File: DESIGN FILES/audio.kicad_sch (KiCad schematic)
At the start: 22 parts, among them J501 PJ-342B-TX-SMT, J502 PJ-342B-TX-SMT, J503 PJ-342B-TX-SMT, U501 WM8978CGEFL_RV

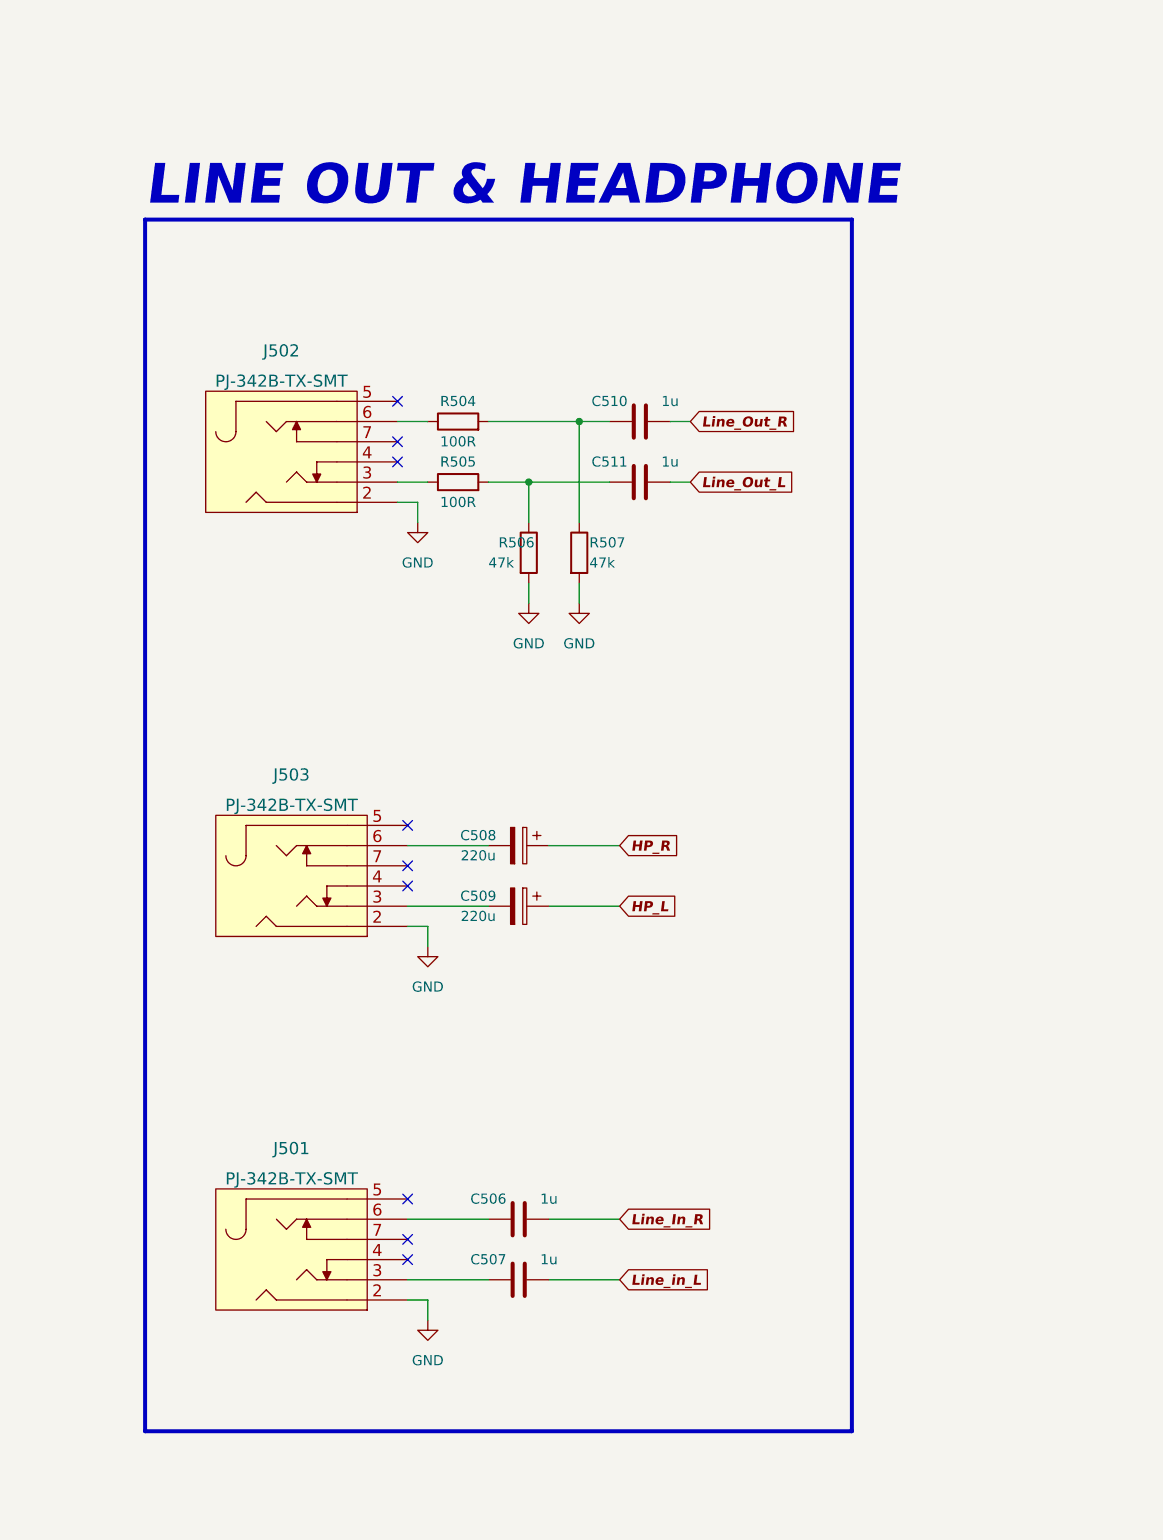
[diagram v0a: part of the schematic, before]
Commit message: updates
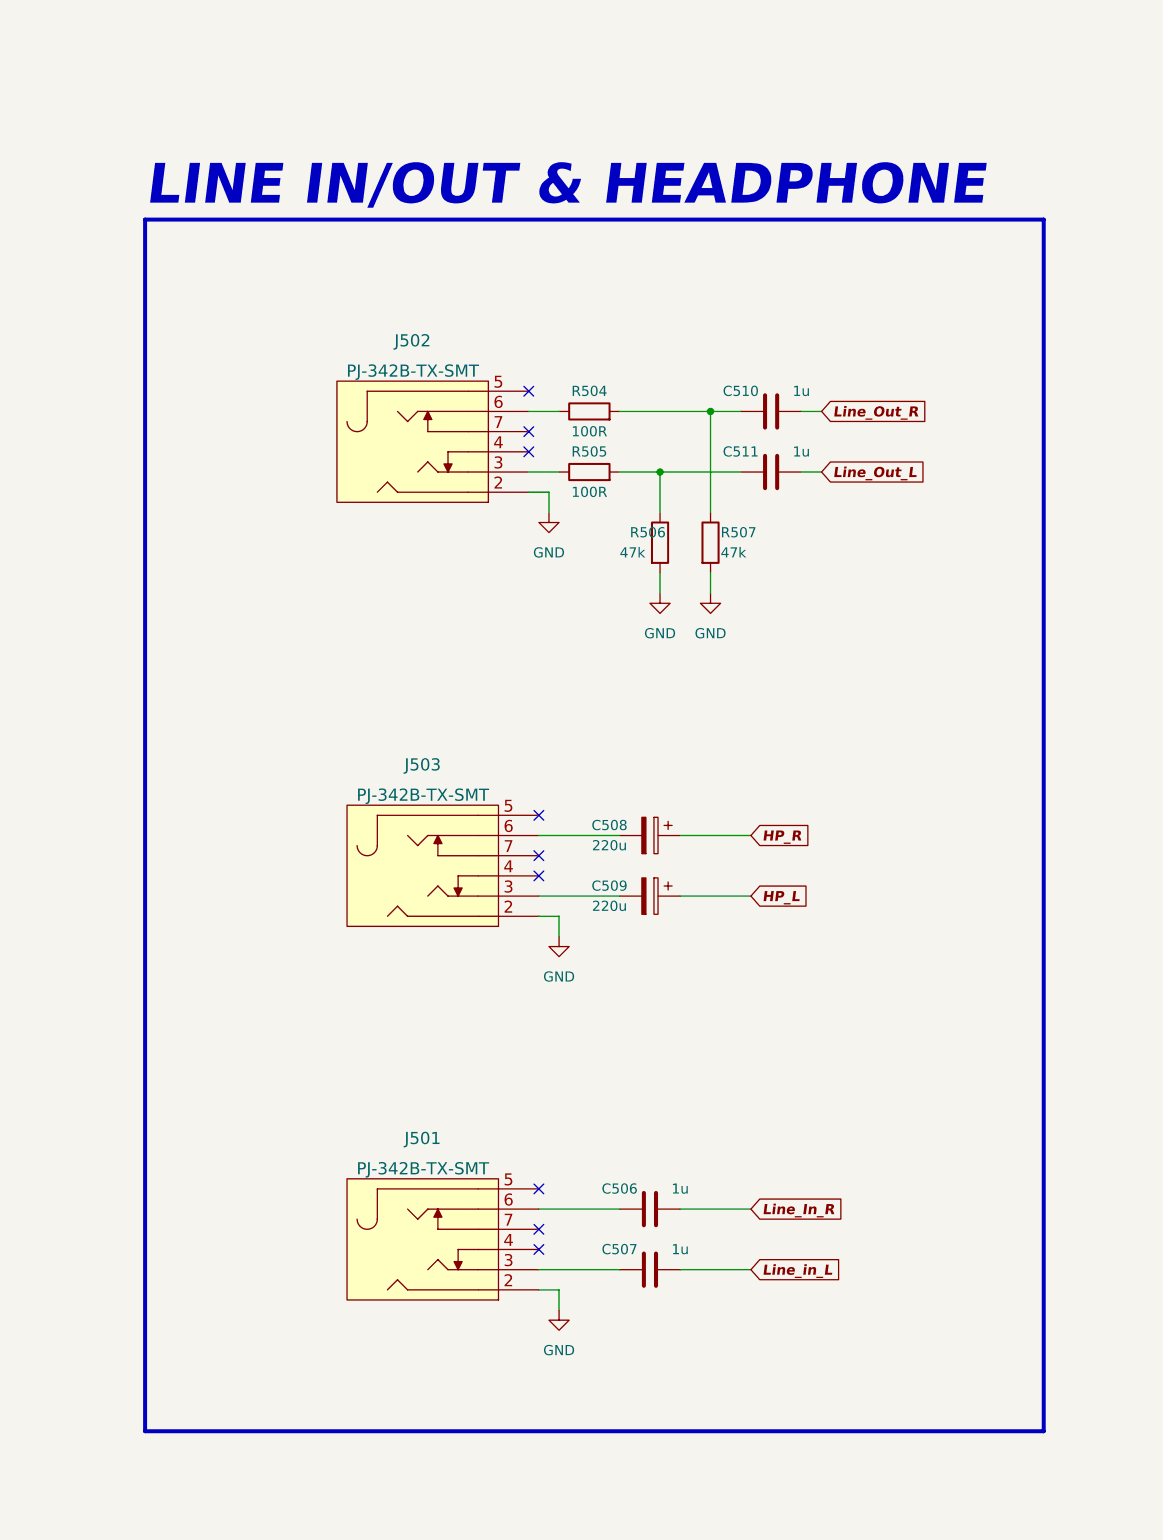
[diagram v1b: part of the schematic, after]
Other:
- note added: "LINE IN/OUT & HEADPHONE"
- note removed: "LINE OUT & HEADPHONE"
- moved on the sheet: C506, C507, C508, C509, C510, C511, J501, J502, J503, R504, R505, R506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
